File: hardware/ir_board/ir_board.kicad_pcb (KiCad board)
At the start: 2 copper layers, 30 x 30 mm, 19 parts, among them J1 Conn_01x04, J2 Conn_01x06, Q1 IRLML0030, U1 VL53L0CXV0DH1

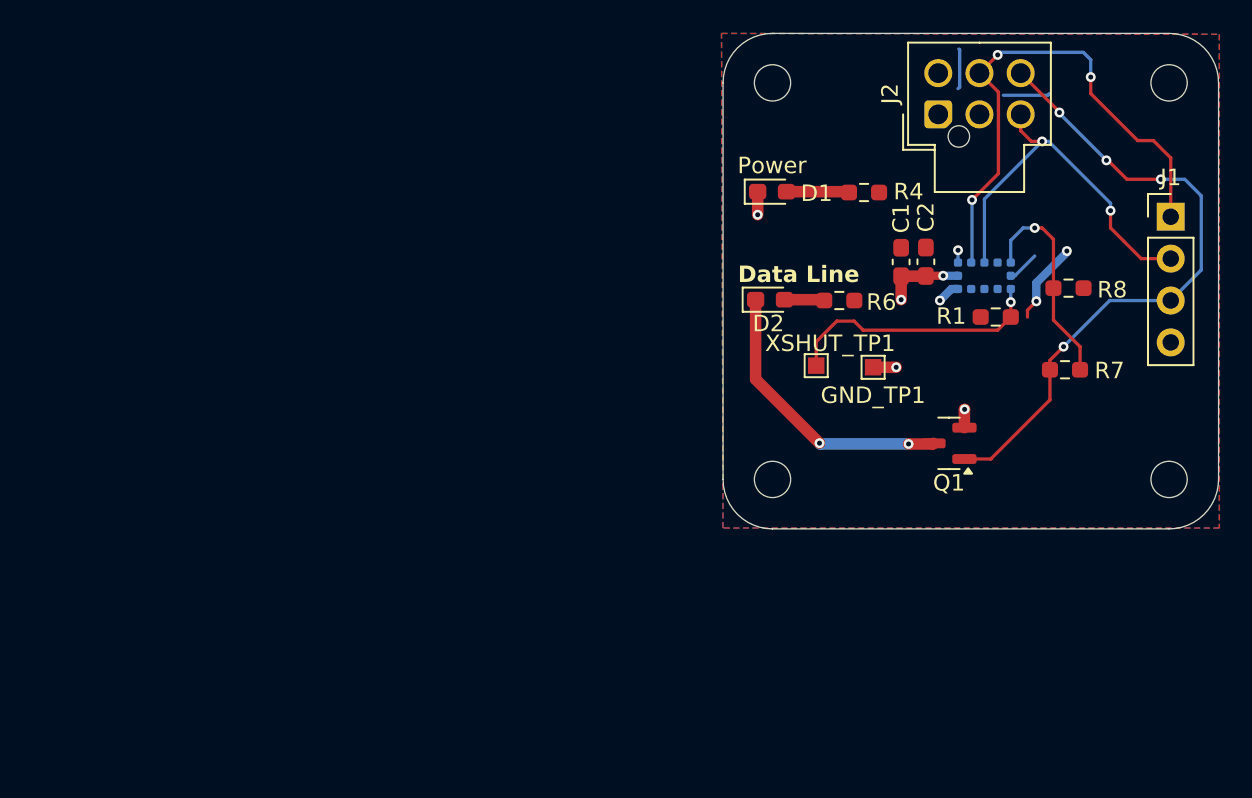
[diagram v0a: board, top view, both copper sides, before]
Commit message: finished irboard, tempboard
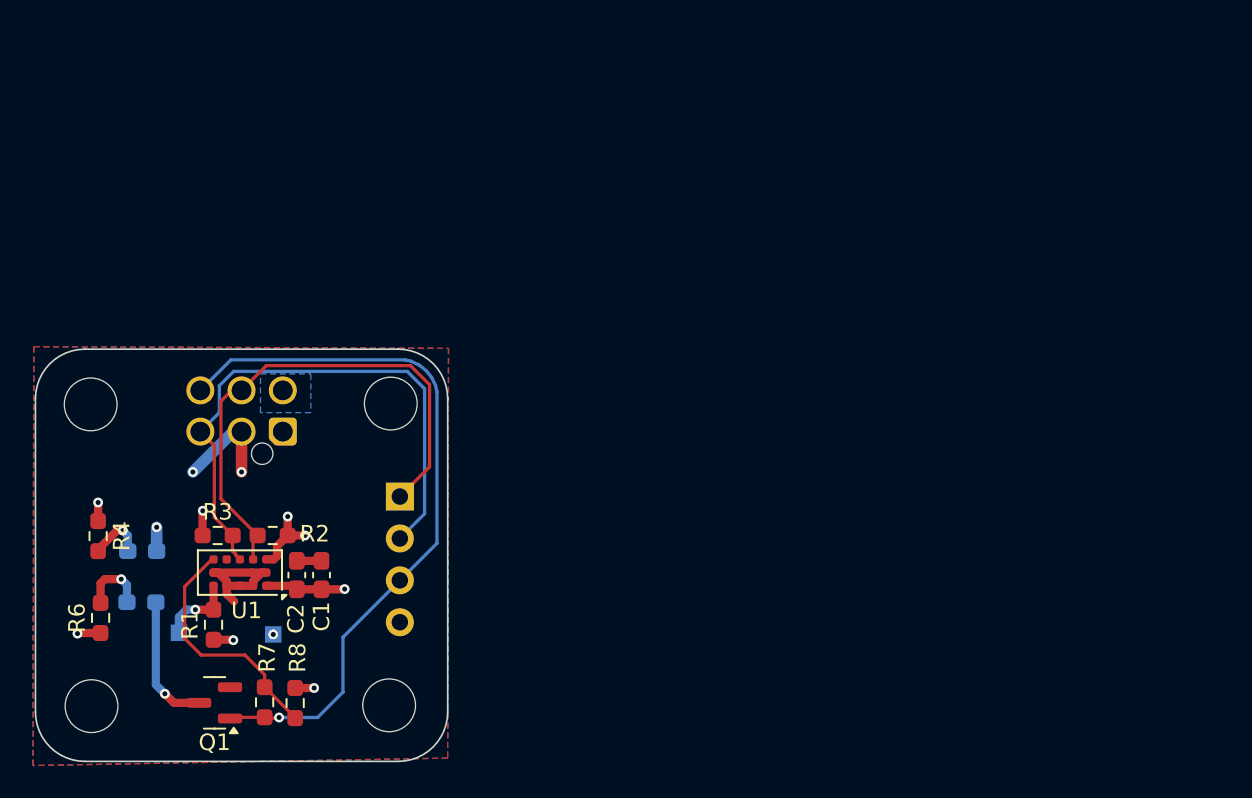
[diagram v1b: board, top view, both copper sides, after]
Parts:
- removed GND_TP1, XSHUT_TP1: TestPoint, TestPoint:TestPoint_Pad_1.0x1.0mm
- added G***: LHRs_LOGO, UTSVT_Logos:LHRs_LOGO, B.Cu at (160.3, 75.9)
- added GND: TestPoint, TestPoint:TestPoint_Pad_1.0x1.0mm, B.Cu at (162.8, 71.5)
- added R2: 4.7k, Resistor_SMD:R_0603_1608Metric_Pad0.98x0.95mm_HandSolder, F.Cu at (162.7, 65.5)
- added R3: 4.7k, Resistor_SMD:R_0603_1608Metric_Pad0.98x0.95mm_HandSolder, F.Cu at (159.4, 65.5)
- added XSHUT: TestPoint, TestPoint:TestPoint_Pad_1.0x1.0mm, B.Cu at (157.1, 71.3)
- D1, D2, J1, J2: moved to B.Cu
- H1, H2, H3, H4: footprint MountingHole:MountingHole_2.2mm_M2 -> MountingHole:MountingHole_3.2mm_M3
- U1: moved to F.Cu
- moved H3 66.8 mm to (151.8, 75.8)
- moved R8 53.2 mm to (164.1, 75.6), turned to -90 degrees
- moved R7 52.6 mm to (162.2, 75.6), turned to 90 degrees
- moved H2 51.1 mm to (169.9, 57.5)
- moved R1 51.0 mm to (159.2, 70.9), turned to 90 degrees
- moved R4 50.9 mm to (152.2, 65.5), turned to -90 degrees
- moved J1 49.7 mm to (170.4, 63.1), turned to 180 degrees
- moved R6 48.8 mm to (152.3, 70.5), turned to 90 degrees
- moved U1 48.6 mm to (160.8, 67.7), turned to 180 degrees
- moved Q1 47.2 mm to (159.2, 75.6)
- moved H1 45.7 mm to (151.7, 57.5)
- moved J2 44.2 mm to (163.3, 59.1)
- moved D1 44.0 mm to (154.8, 66.4), turned to 180 degrees
- moved C2 42.6 mm to (164.2, 67.8), turned to 90 degrees
- moved D2 42.3 mm to (154.8, 69.5), turned to 180 degrees
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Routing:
- net /SDA: track 23.0 -> 35.0 mm, vias 2 -> 0
- net /XSHUT: track 16.0 -> 4.69 mm
- net Net-(D2-K): track 17.3 -> 8.22 mm, vias 2 -> 1
- net +3.3V: track 7.13 -> 15.7 mm, vias 4 -> 8
- net /GPIO1: track 39.1 -> 44.2 mm, vias 4 -> 1
- net Net-(D2-A): track 2.43 -> 4.09 mm, vias 0 -> 1
- net Net-(U1-GPIO1): track 13.1 -> 14.7 mm, vias 1 -> 0
- net GND: track 16.1 -> 17.6 mm, vias 5 -> 4
- net Net-(D1-A): track 3.81 -> 3.45 mm, vias 0 -> 1
- net /SCL: vias 3 -> 0
- added copper zone on B.Cu, net +3.3V
- added copper zone on F.Cu, net GND
- removed copper zone on F.Cu, net +3.3V
- removed copper zone on B.Cu, net GND
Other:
- board size 30 x 30 mm -> 25 x 25 mm
- board text added: "Data"
- board text removed: "Data Line"
